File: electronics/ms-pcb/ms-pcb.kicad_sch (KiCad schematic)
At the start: 25 parts, among them J1 Left motor, J2 Right motor, J3 XT60-M, U1 ESP32-S3-DEVKITC-1U-N8R2, U2 GY-521

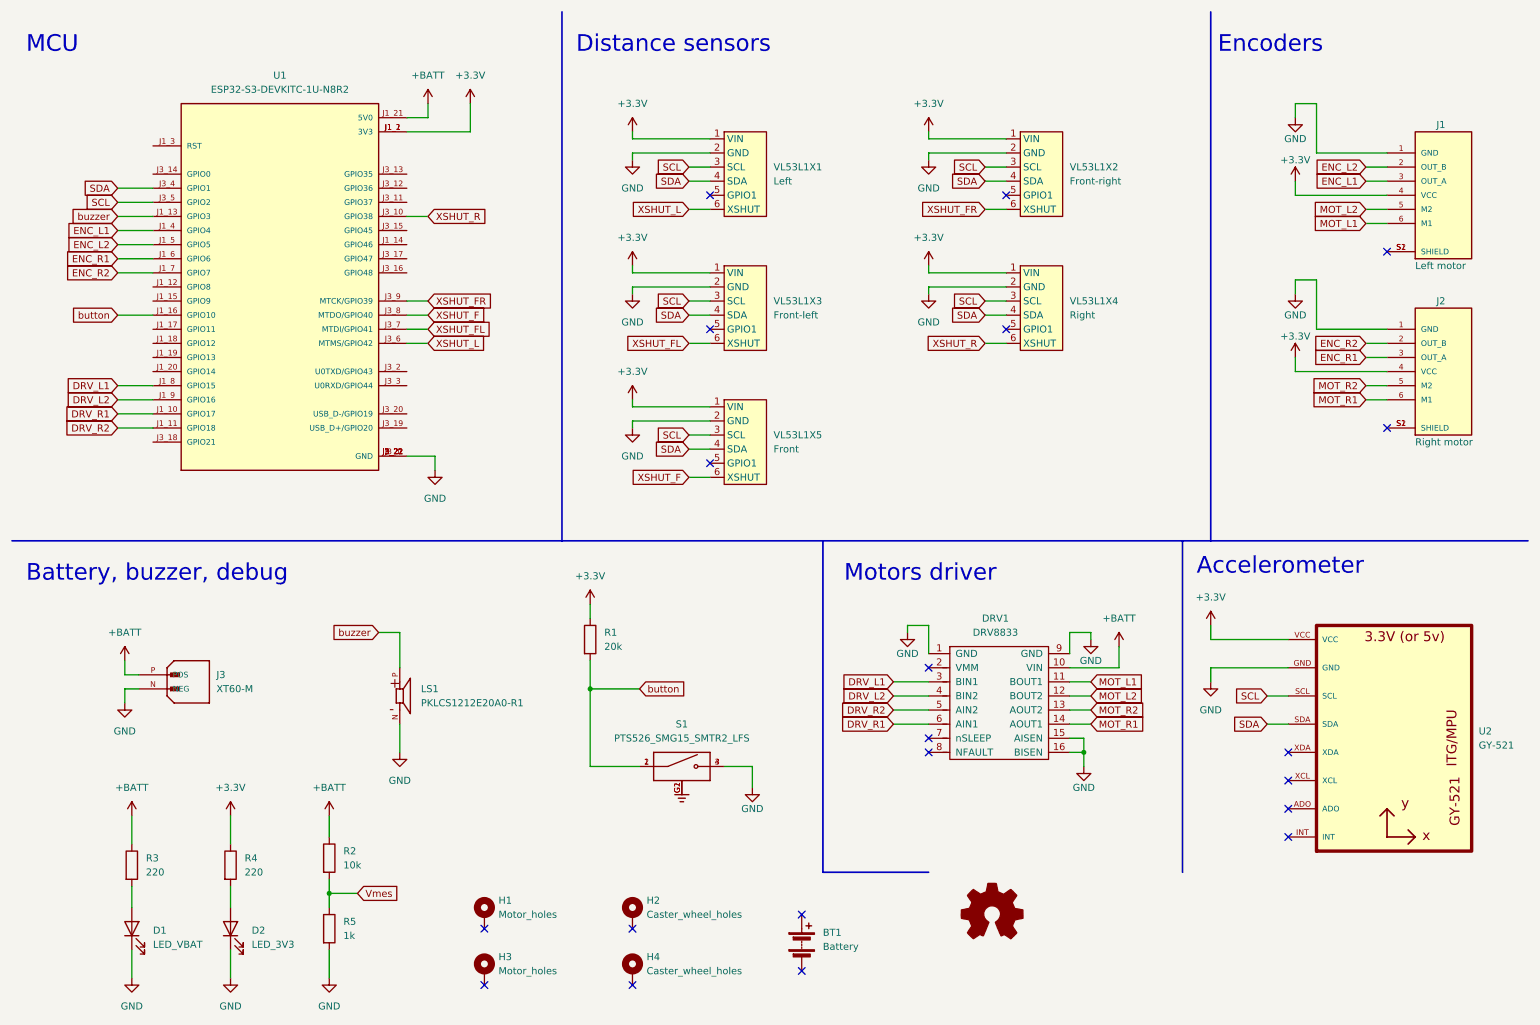
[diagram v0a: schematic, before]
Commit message: elec: PCB layout wiring
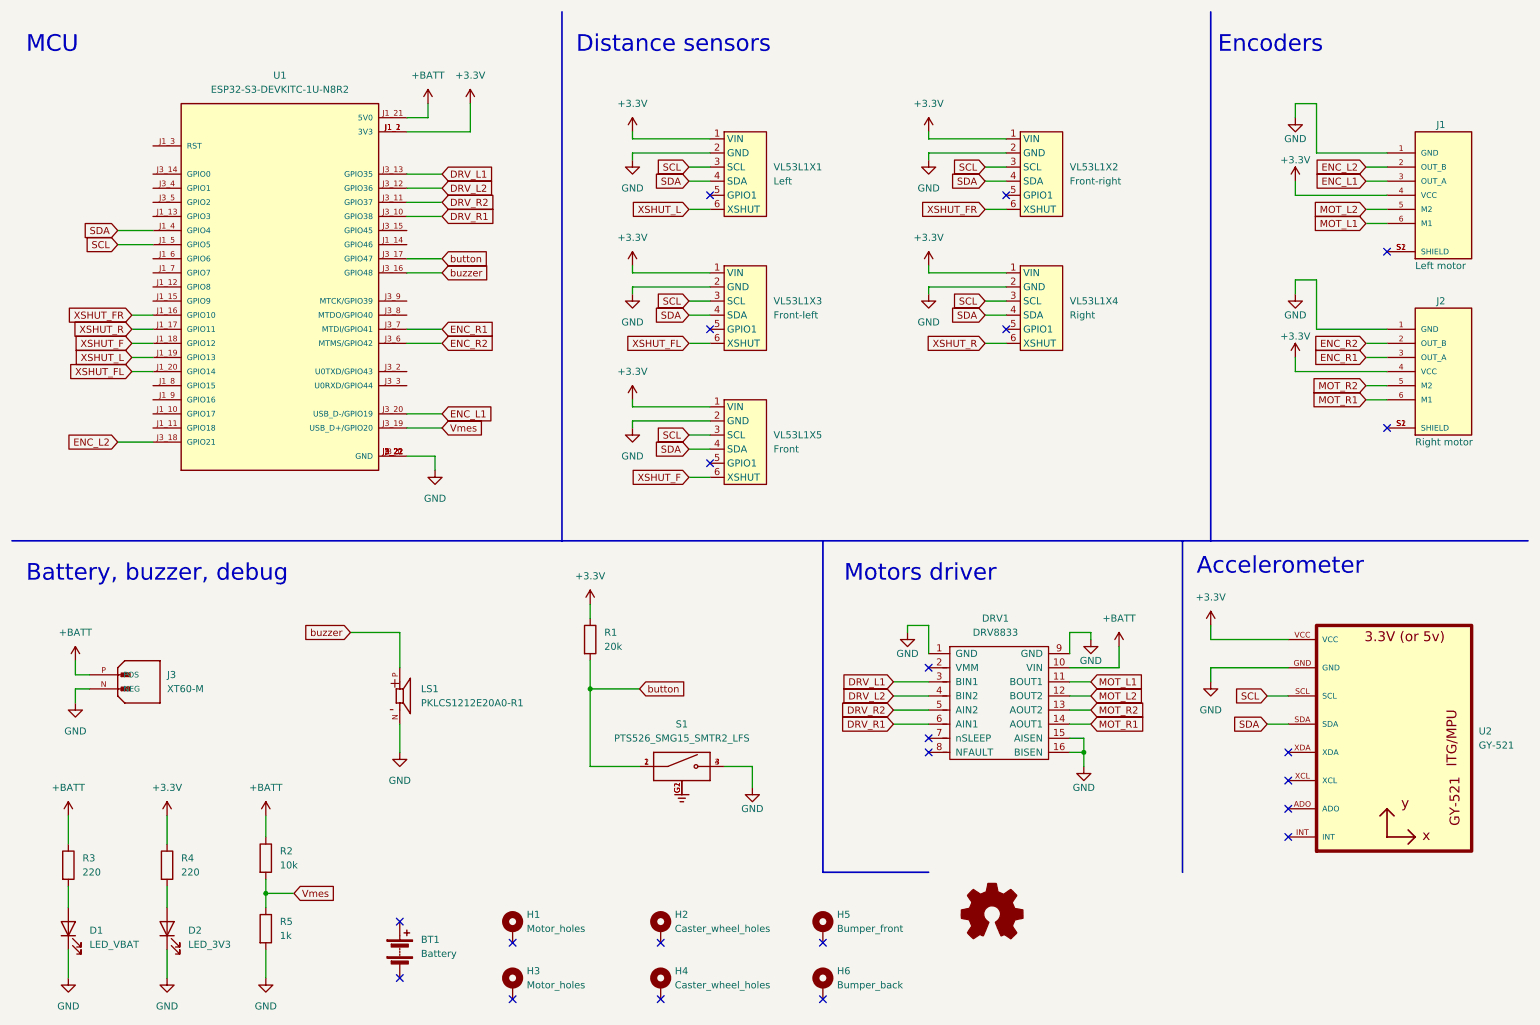
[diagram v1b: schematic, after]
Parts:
- added H5: Bumper_front, footprints:Micromouse_bumper, symbol Mechanical:MountingHole_Pad
- added H6: Bumper_back, footprints:Micromouse_bumper, symbol Mechanical:MountingHole_Pad
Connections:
- net DRV_L1: now also U1.J3_13 (GPIO35); no longer U1.J1_8 (GPIO15)
- net DRV_L2: now also U1.J3_12 (GPIO36); no longer U1.J1_9 (GPIO16)
- net DRV_R1: now also U1.J3_10 (GPIO38); no longer U1.J1_10 (GPIO17)
- net DRV_R2: now also U1.J3_11 (GPIO37); no longer U1.J1_11 (GPIO18)
- net ENC_L1: now also U1.J3_20 (USB_D-/GPIO19); no longer U1.J1_4 (GPIO4)
- net ENC_L2: now also U1.J3_18 (GPIO21); no longer U1.J1_5 (GPIO5)
- net ENC_R1: now also U1.J3_7 (MTDI/GPIO41); no longer U1.J1_6 (GPIO6)
- net ENC_R2: now also U1.J3_6 (MTMS/GPIO42); no longer U1.J1_7 (GPIO7)
- net SCL: now also U1.J1_5 (GPIO5); no longer U1.J3_5 (GPIO2)
- net SDA: now also U1.J1_4 (GPIO4); no longer U1.J3_4 (GPIO1)
- net Vmes: now also U1.J3_19 (USB_D+/GPIO20)
- net XSHUT_F: now also U1.J1_18 (GPIO12); no longer U1.J3_8 (MTDO/GPIO40)
- net XSHUT_FL: now also U1.J1_20 (GPIO14); no longer U1.J3_7 (MTDI/GPIO41)
- net XSHUT_FR: now also U1.J1_16 (GPIO10); no longer U1.J3_9 (MTCK/GPIO39)
- net XSHUT_L: now also U1.J1_19 (GPIO13); no longer U1.J3_6 (MTMS/GPIO42)
- net XSHUT_R: now also U1.J1_17 (GPIO11); no longer U1.J3_10 (GPIO38)
- net button: now also U1.J3_17 (GPIO47); no longer U1.J1_16 (GPIO10)
- net buzzer: now also U1.J3_16 (GPIO48); no longer U1.J1_13 (GPIO3)
- no-connect marks 20 -> 22
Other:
- moved on the sheet: BT1, D1, D2, H1, H2, H3, H4, J3, R2, R3, R4, R5
